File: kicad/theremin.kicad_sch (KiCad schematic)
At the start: 40 parts, among them J1 Eurorack Mono Jack, J2 Aerial, SW1 SW_SPDT, U1 4069, U2 4069, U3 LM386, U4 LP2950-5.0_TO92

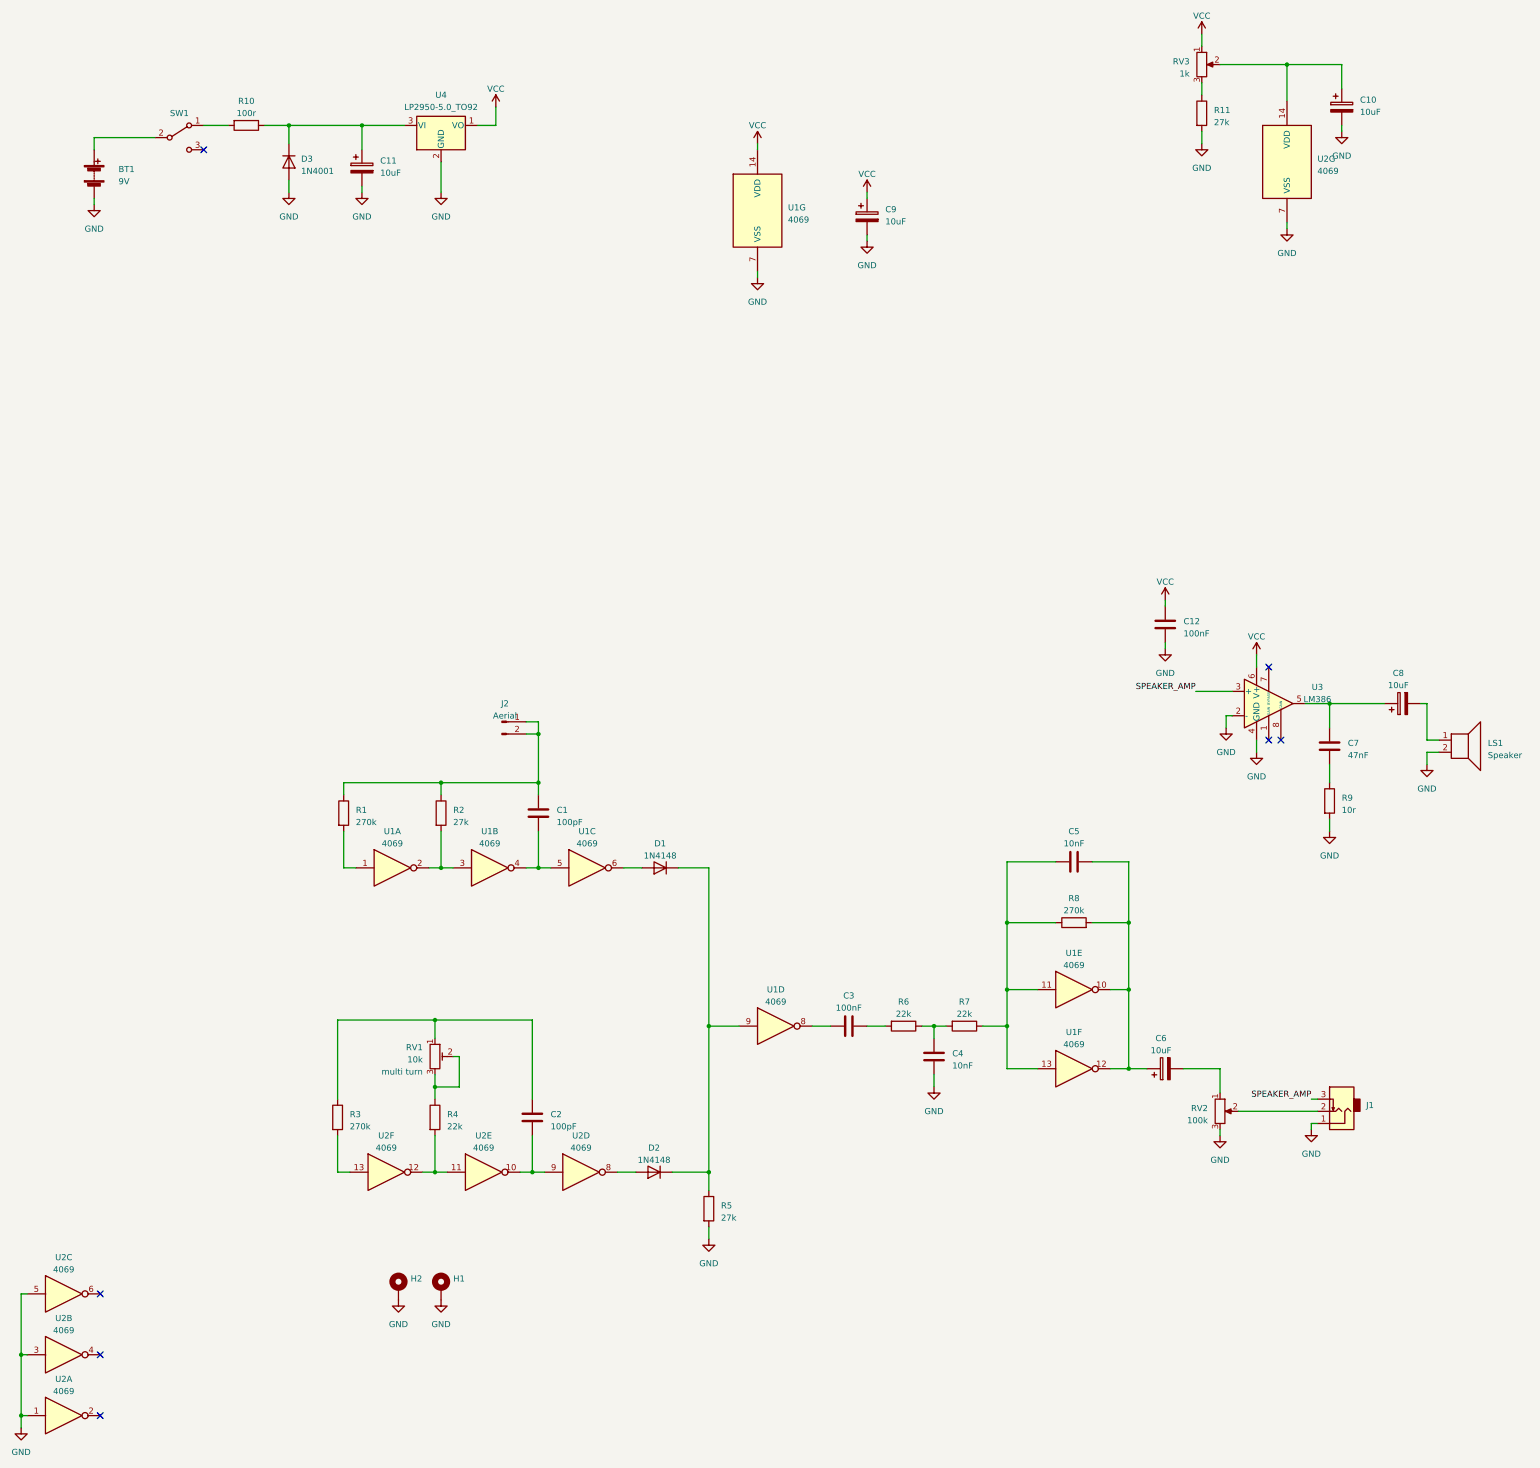
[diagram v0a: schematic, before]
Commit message: Updating with new footprints and some tweaks
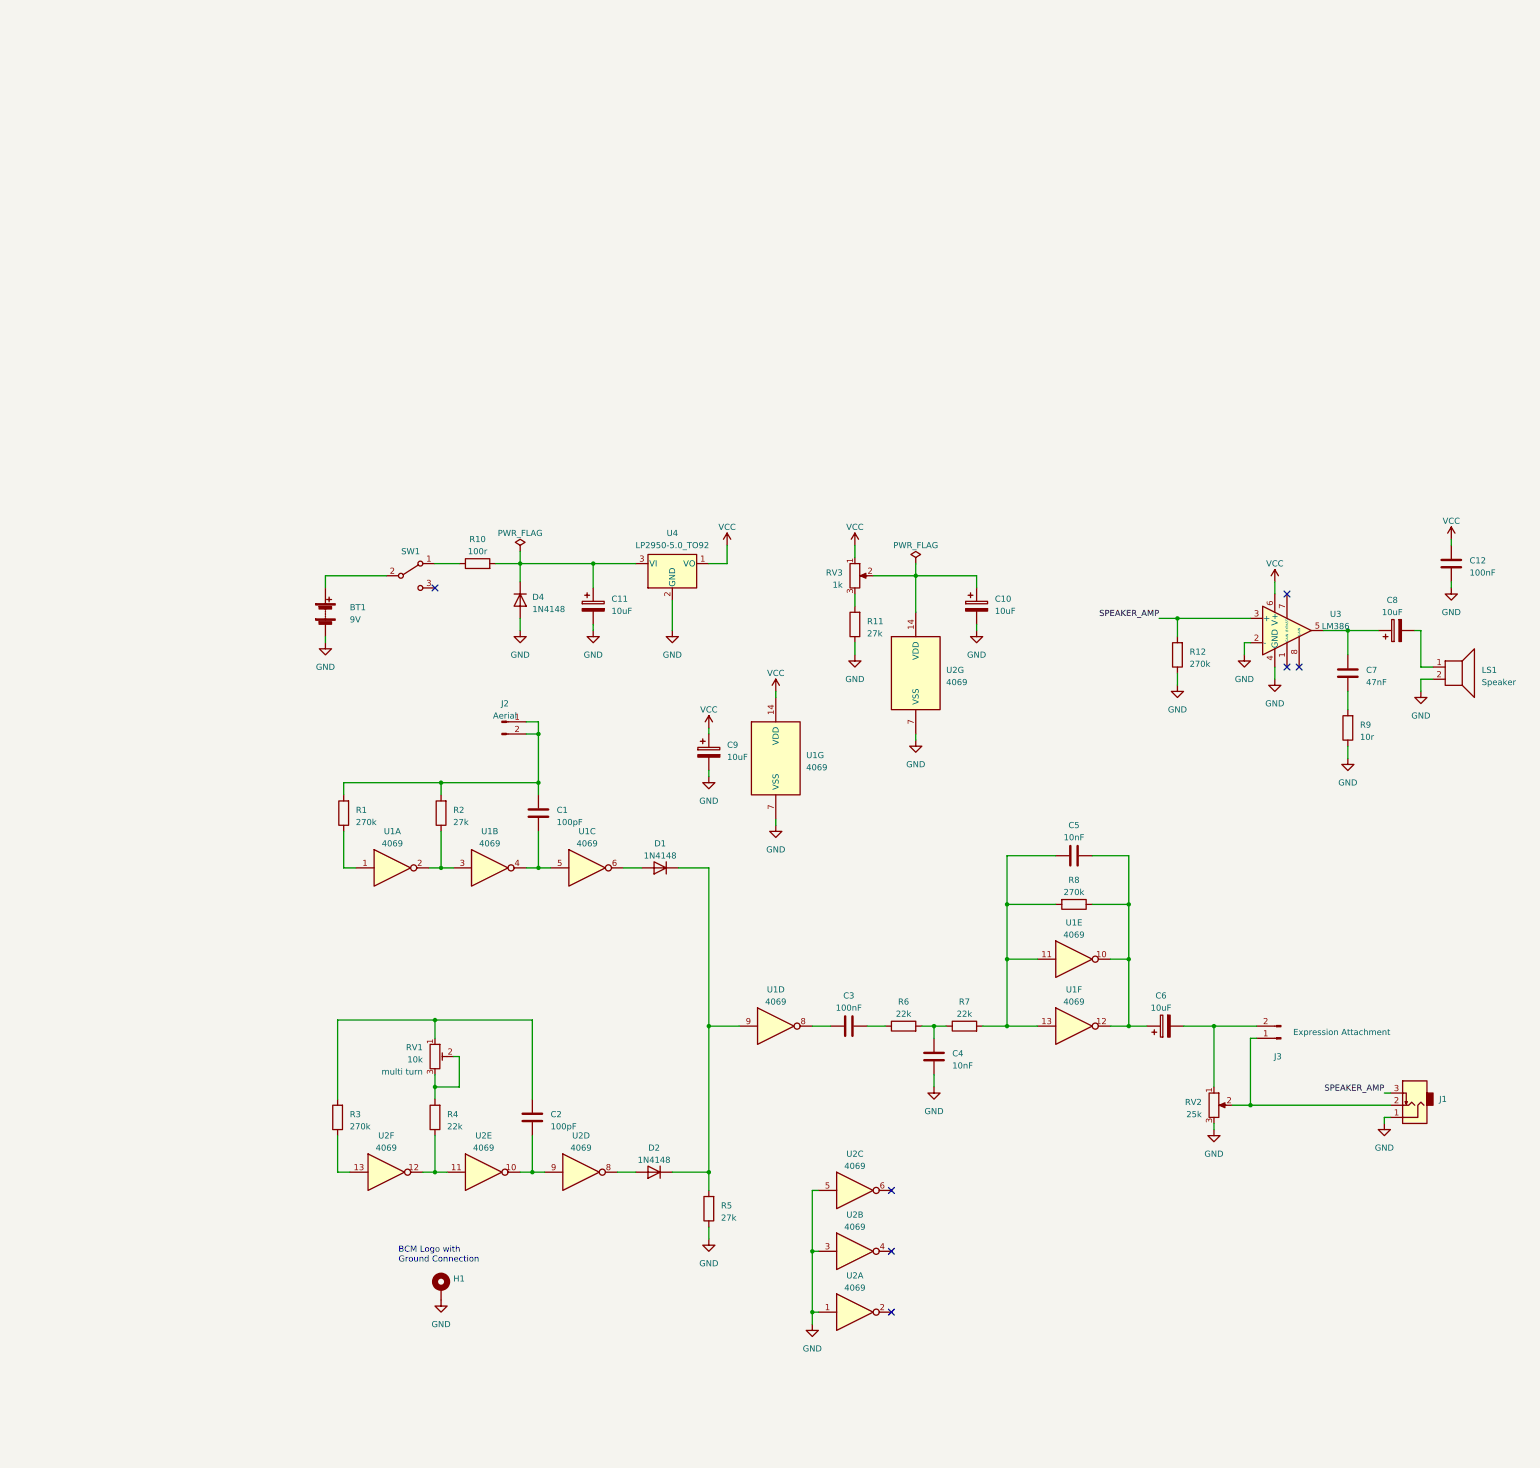
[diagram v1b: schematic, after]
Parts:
- removed D3: 1N4001, Diode_THT:D_DO-35_SOD27_P7.62mm_Horizontal, symbol Diode:1N4148
- removed H2: MountingHole_Pad, MountingHole:MountingHole_3.2mm_M3_DIN965_Pad, symbol Mechanical:MountingHole_Pad
- added D4: 1N4148, Diode_THT:D_DO-35_SOD27_P7.62mm_Horizontal, symbol Diode:1N4148
- added J3: Expression Attachment, Connector_PinHeader_2.54mm:PinHeader_1x02_P2.54mm_Vertical, symbol Connector:Conn_01x02_Pin
- added R12: 270k, Resistor_THT:R_Axial_DIN0207_L6.3mm_D2.5mm_P10.16mm_Horizontal, symbol Device:R
- BT1: footprint Connector_PinHeader_2.54mm:PinHeader_1x02_P2.54mm_Vertical -> Battery:BatteryHolder_Eagle_12BH611-GR
- C1, C2: footprint Rumblesan_Standard_Parts:C_Rect_L7.0mm_W3.5mm_P5.00mm -> Capacitor_THT:C_Rect_L7.0mm_W3.5mm_P5.00mm; Spec (none) -> ceramic C0G; Tolerance (none) -> 1%
- C10, C11, C6, C8, C9: footprint Rumblesan_Standard_Parts:CP_Radial_D5.0mm_P2.00mm -> Capacitor_THT:CP_Radial_D5.0mm_P2.50mm; symbol Rumblesan Standard Parts:C_Polarized -> Device:C_Polarized
- C12: footprint Rumblesan_Standard_Parts:C_Rect_L7.0mm_W3.5mm_P5.00mm -> Capacitor_THT:C_Rect_L7.0mm_W3.5mm_P5.00mm; symbol Rumblesan Standard Parts:C -> Device:C; Spec ceramic C0G -> ceramic X7R
- C3, C4, C5, C7: footprint Rumblesan_Standard_Parts:C_Rect_L7.0mm_W3.5mm_P5.00mm -> Capacitor_THT:C_Rect_L7.0mm_W3.5mm_P5.00mm; symbol Rumblesan Standard Parts:C -> Device:C
- H1: footprint MountingHole:MountingHole_3.2mm_M3_DIN965_Pad -> project-footprints:BCM_Logo_small_Copper_Pad_15mmx15mm; now left out of the parts list
- J2: now left out of the parts list
- LS1: footprint Connector_PinHeader_2.54mm:PinHeader_1x02_P2.54mm_Vertical -> project-footprints:Speaker_PUIAudio_AS04008MR-21-R
- R1, R10, R11, R2, R3, R4, R5, R6, R7, R8, R9: footprint Rumblesan_Standard_Parts:R_Axial_DIN0207_L6.3mm_D2.5mm_P10.16mm_Horizontal -> Resistor_THT:R_Axial_DIN0207_L6.3mm_D2.5mm_P10.16mm_Horizontal; symbol Rumblesan Standard Parts:R -> Device:R
- RV2: value 100k -> 25k; footprint Rumblesan_Standard_Parts:Potentiometer_Alpha_RD901F-40-00D_Single_Vertical -> Potentiometer_THT:Potentiometer_Alpha_RD901F-40-00D_Single_Vertical
- RV3: footprint Rumblesan_Standard_Parts:Potentiometer_Alpha_RD901F-40-00D_Single_Vertical -> Potentiometer_THT:Potentiometer_Alpha_RD901F-40-00D_Single_Vertical
- SW1: footprint Rumblesan_Standard_Parts:SW_SPDT_DailyWell_Sub_MiniToggle -> Button_Switch_THT:SW_CuK_OS102011MA1QN1_SPDT_Angled; MPRN (none) -> OS102011MA1QN1
- U1, U2: footprint Rumblesan_Standard_Parts:DIP-14_W7.62mm_Socket -> Package_DIP:DIP-14_W7.62mm_Socket_LongPads
- U3: footprint Rumblesan_Standard_Parts:DIP-8_W7.62mm_Socket -> Package_DIP:DIP-8_W7.62mm_Socket_LongPads
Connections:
- net GND: now also R11.1, R5.1, R9.1, D4.2 (A), R12.1; no longer R11.2, R5.2, R9.2
- net SPEAKER_AMP: now also R12.2
- net at U1.1: now also R1.1; no longer R1.2
- net at U1.2, U1.3: now also R2.1; no longer R2.2
- net at C5.2, U1.11, U1.13: now also R7.2, R8.2; no longer R7.1, R8.1
- net at U2.10, U2.9: now also C2.1; no longer C2.2
- net at R6.2: now also C4.2, R7.1; no longer C3.2
- net at U2.11, U2.12: now also R4.1; no longer R4.2
- net at U2.13: now also R3.1; no longer R3.2
- net at D1.1 (K), D2.1 (K), U1.9: now also R5.2; no longer R5.1
- net at J1.2 (Tip), RV2.2: now also J3.1 (Pin_1)
- net at U1.4, U1.5: now also C1.1; no longer C1.2
- net at C5.1, C6.1, U1.10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: now also R8.1; no longer R8.2
- net at RV3.3: now also R11.2; no longer R11.1
- net at C11.1, U4.3 (VI): now also R10.2, D4.1 (K); no longer R10.1
- net at RV1.2, RV1.3: now also R4.2; no longer R4.1
- net at C6.2, RV2.1: now also J3.2 (Pin_2)
- net at C7.1: now also R9.2; no longer R9.1
- net at SW1.1 (A): now also R10.1; no longer R10.2
- new net: C1.2, J2.1 (Pin_1), J2.2 (Pin_2), R1.2, R2.2
- new net: C3.2, R6.1
- new net: C2.2, R3.2, RV1.1
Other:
- note added: "BCM Logo with Ground Connection"
- moved on the sheet: BT1, C10, C11, C12, C5, C6, C7, C8, C9, J1, LS1, R10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
